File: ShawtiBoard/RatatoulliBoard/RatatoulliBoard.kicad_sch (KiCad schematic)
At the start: 52 parts, among them IC1 TEENSY_4.1, IC2 DRV8212DRLR, IC3 DRV8212DRLR, J1 BDC1, J2 BDC2, J3 LIDAR1, J4 LIDAR2, J5 LIDAR3, J6 LIDAR4, J7 LINE_RF, J8 LINE_LF, J9 Battery, SW1 SW_DIP_x03, SW2 SW_SPST, U1 ADP2303ARDZ-R7, U2 ADP2303ARDZ-R7

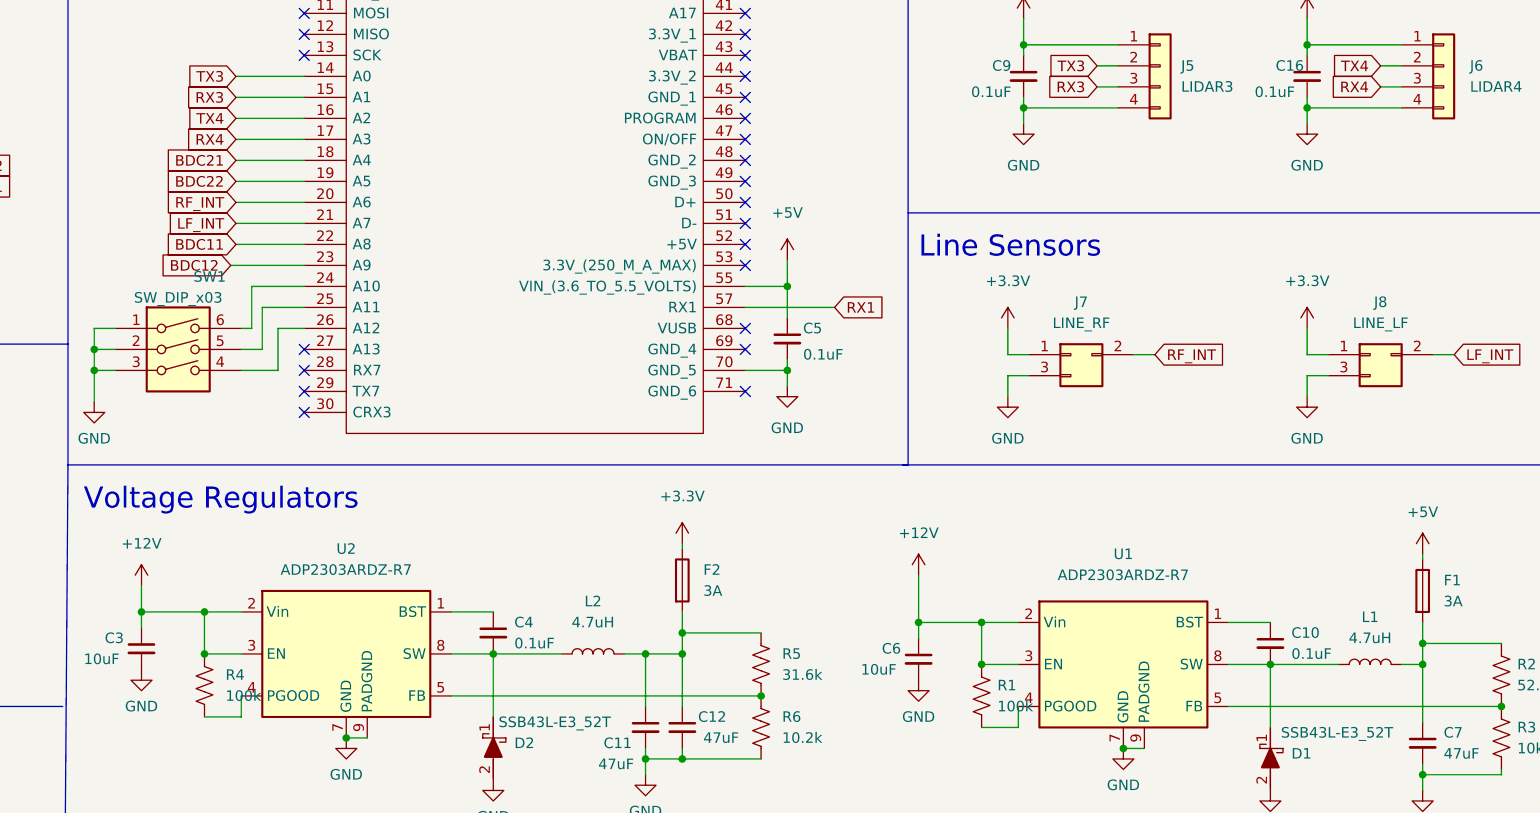
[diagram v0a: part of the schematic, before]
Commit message: Spedrun board layout
minor edits to schematic for layout purposes. finally finished layout for manufacturing
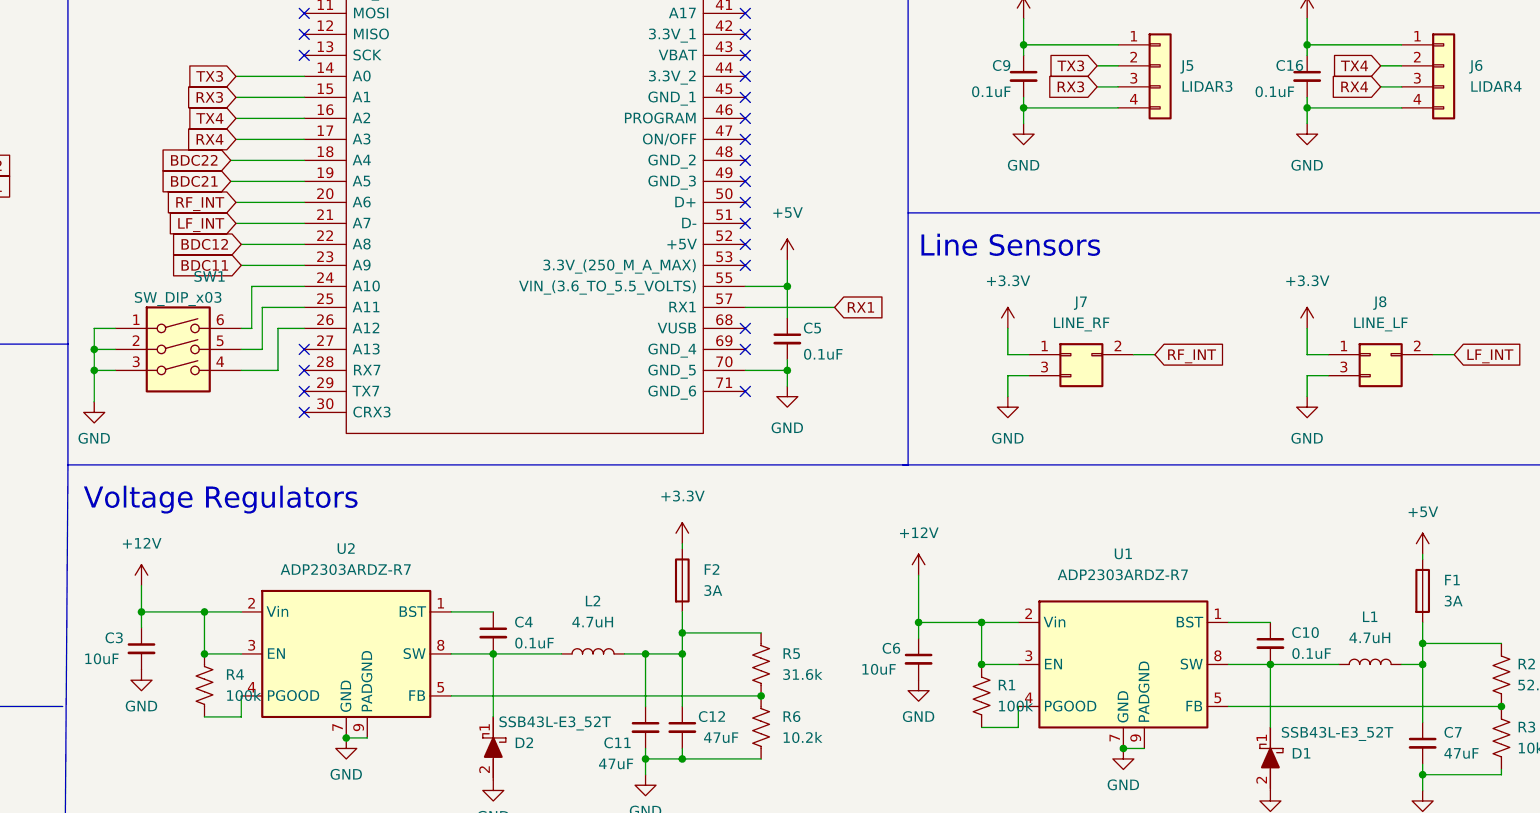
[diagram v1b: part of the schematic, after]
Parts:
- R9: footprint kicadLib:C_0402_1005Metric -> Diode_SMD:D_0805_2012Metric
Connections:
- net BDC11: now also IC1.23 (A9); no longer IC1.22 (A8)
- net BDC12: now also IC1.22 (A8); no longer IC1.23 (A9)
- net BDC21: now also IC1.19 (A5); no longer IC1.18 (A4)
- net BDC22: now also IC1.18 (A4); no longer IC1.19 (A5)
